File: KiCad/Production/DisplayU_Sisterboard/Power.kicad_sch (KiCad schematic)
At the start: 16 parts, among them Q2 AO3421E, U3 AP2112K-3.3TRG1

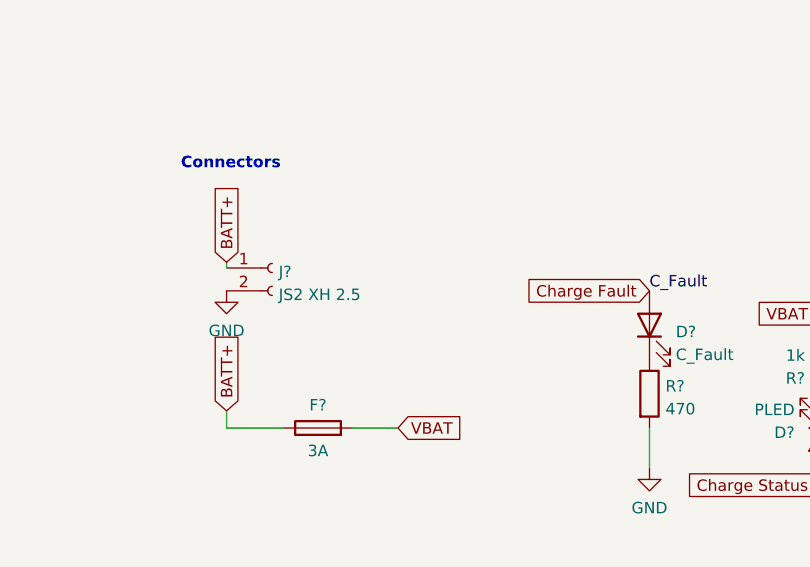
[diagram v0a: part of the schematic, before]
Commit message: Berekening/Metingen Verslag
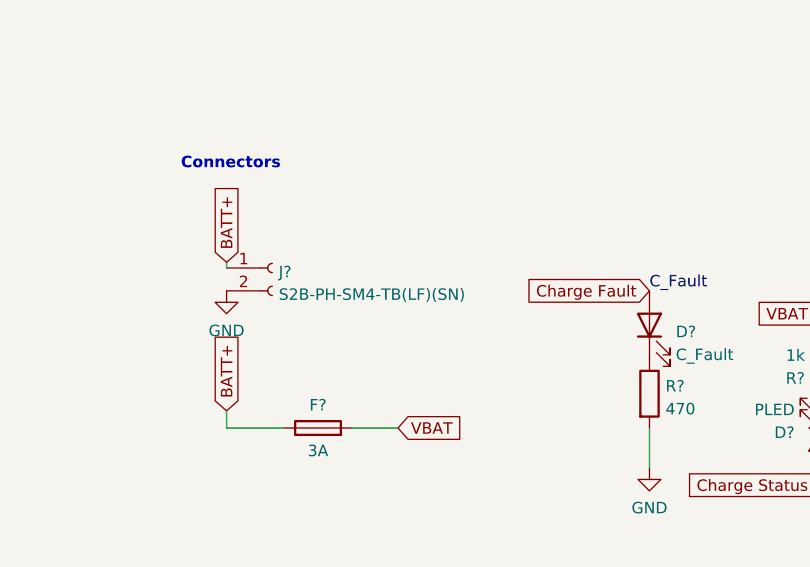
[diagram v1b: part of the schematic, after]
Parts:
- J?: value JS2 XH 2.5 -> S2B-PH-SM4-TB(LF)(SN)
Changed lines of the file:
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@@
   (symbol (lib_id "Connector:Conn_01x02_Female") (at 91.44 62.23 0) (unit 1)
     (in_bom yes) (on_board yes) (dnp no) (fields_autoplaced)
-    (property "Reference" "J?" (at 92.1512 62.6653 0)
+    (property "Reference" "J?" (at 92.1512 62.6752 0)
       (effects (font (size 1.27 1.27)) (justify left))
     )
-    (property "Value" "JS2 XH 2.5" (at 92.1512 65.2022 0)
+    (property "Value" "S2B-PH-SM4-TB(LF)(SN)" (at 92.1512 65.1804 0)
       (effects (font (size 1.27 1.27)) (justify left))
     )
